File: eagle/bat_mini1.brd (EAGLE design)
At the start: 79.2 x 86.4 mm, 13 parts

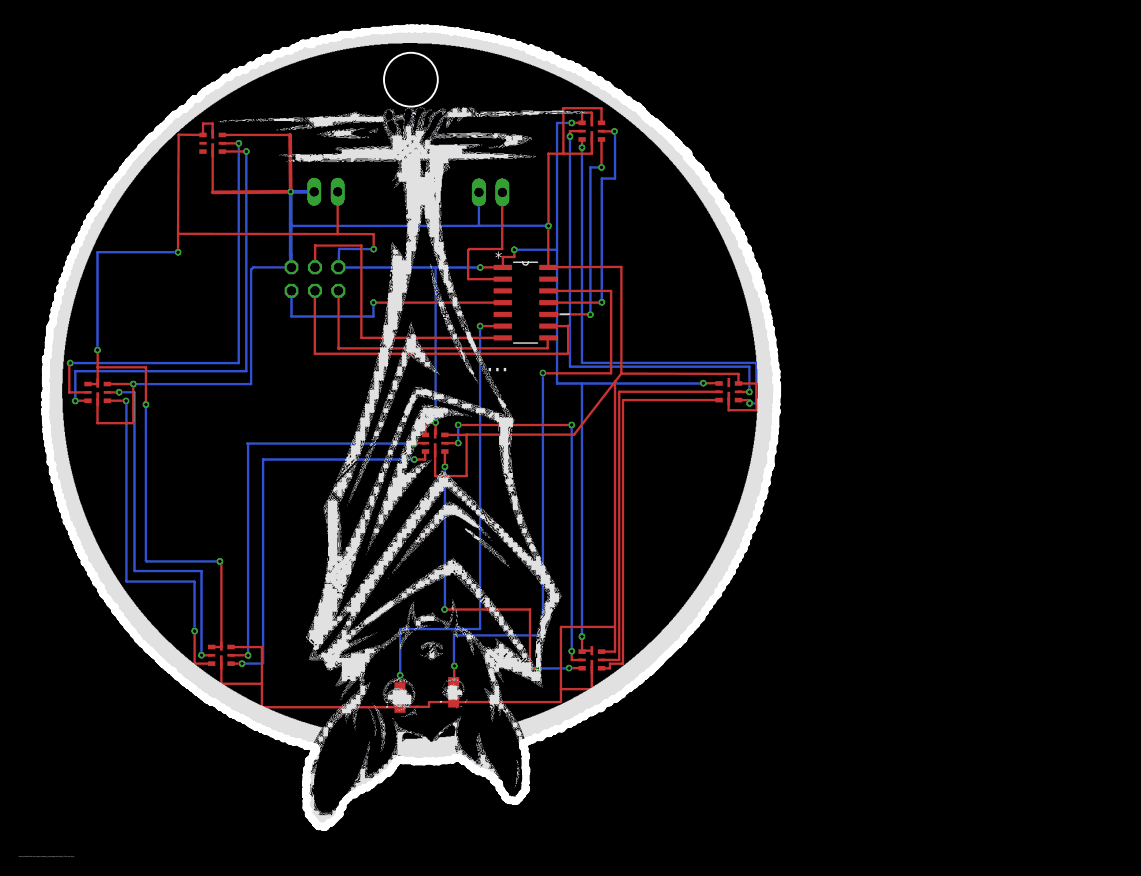
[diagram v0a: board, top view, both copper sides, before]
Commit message: post proto updates
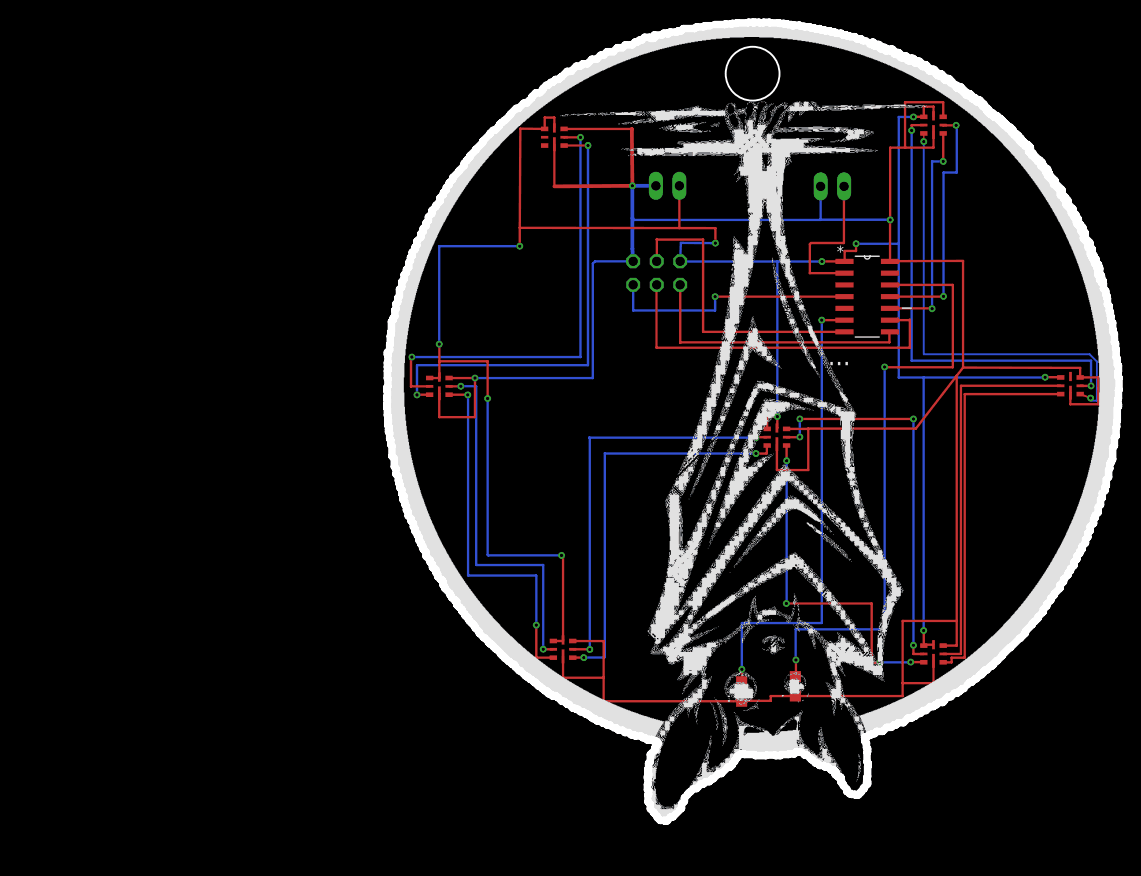
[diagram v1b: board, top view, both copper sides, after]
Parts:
- moved . 37.0 mm to (84.0, 18.1)
- moved .. 37.0 mm to (78.2, 17.6)
- moved DEBUG 37.0 mm to (88.0, 72.2)
- moved EYE1 37.0 mm to (99.0, 78.8)
- moved EYE2 37.0 mm to (113.8, 50.6)
- moved ISP 37.0 mm to (69.0, 62.8)
- moved POWER 37.0 mm to (70.2, 72.3)
- moved U$4 37.0 mm to (99.0, 21.6)
- moved U$5 37.0 mm to (82.0, 45.1)
- moved U$6 37.0 mm to (58.9, 22.1)
- moved U$7 37.0 mm to (45.5, 50.6)
- moved U$8 37.0 mm to (58.0, 77.5)
- moved ... 37.0 mm to (91.8, 60.3)
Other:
- outline, holes or cut-outs redrawn
- board text removed: "/home/thedevilsvoice/workspace/badge_proto/batgoth/art/bat_silkscreen.bmp"
- board text removed: "DE:AD:10:C5 @mzbat @theDevilsVoice @p0lr_"
